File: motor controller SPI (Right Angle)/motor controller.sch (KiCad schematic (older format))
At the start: 27 parts, among them IC1 MA702, IC2 MC33926PNB, IC3 LP38690SD-ADJ_NOPB, J1 Conn_01x06_Male, J2 Conn_01x06_Male, J3 Conn_01x04_Male, M1 Motor_DC, U1 STM32L432KCUx, Y1 32mhz

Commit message: Updated footprints
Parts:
- removed C1, C2: 10pF, Capacitor_SMD:C_0402_1005Metric, symbol Device:C
- removed IC3: LP38690SD-ADJ_NOPB, LP38690SD-ADJ_NOPB:SON95P300X300X80-7N, symbol LP38690SD-ADJ_NOPB:LP38690SD-ADJ_NOPB
- removed Y1: 32mhz, Crystal:Crystal_SMD_2016-4Pin_2.0x1.6mm, symbol Device:Crystal_GND24
- added U2: MIC5501-3.0YM5, Package_TO_SOT_SMD:SOT-23-5, symbol Regulator_Linear:MIC5501-3.0YM5
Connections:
- wire segments 36 -> 28
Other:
- moved on the sheet: C9
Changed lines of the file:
@@
-$EndComp
-$Comp
-L Device:C C1
-U 1 1 5B480489
-P 1000 2650
-F 0 "C1" V 748 2650 50  0000 C CNN
-F 1 "10pF" V 839 2650 50  0000 C CNN
-F 2 "Capacitor_SMD:C_0402_1005Metric" H 1038 2500 50  0001 C CNN
-F 3 "~" H 1000 2650 50  0001 C CNN
-	1    1000 2650
-	0    1    1    0
-$EndComp
-$Comp
-L Device:C C2
-U 1 1 5B480490
-P 1000 2950
-F 0 "C2" V 1252 2950 50  0000 C CNN
-F 1 "10pF" V 1161 2950 50  0000 C CNN
-F 2 "Capacitor_SMD:C_0402_1005Metric" H 1038 2800 50  0001 C CNN
-F 3 "~" H 1000 2950 50  0001 C CNN
-	1    1000 2950
-	0    -1   -1   0
-$EndComp
-Wire Wire Line
-	850  2650 850  2800
-Wire Wire Line
-	1150 2650 1300 2650
-Wire Wire Line
-	1150 2950 1300 2950
-Connection ~ 1300 2950
-Connection ~ 1300 2650
-$Comp
-L power:GND #PWR0101
-U 1 1 5B4804A2
-P 850 2800
-F 0 "#PWR0101" H 850 2550 50  0001 C CNN
-F 1 "GND" V 855 2672 50  0000 R CNN
-F 2 "" H 850 2800 50  0001 C CNN
-F 3 "" H 850 2800 50  0001 C CNN
-	1    850  2800
-	0    1    1    0
-$EndComp
-Connection ~ 850  2800
-Wire Wire Line
-	850  2800 850  2950
-Wire Wire Line
-	1300 2950 2050 2950
-Wire Wire Line
-	1550 2850 2050 2850
-Wire Wire Line
-	1550 2650 1550 2850
-$Comp
-L power:GND #PWR0102
-U 1 1 5B487486
-P 1600 2650
-F 0 "#PWR0102" H 1600 2400 50  0001 C CNN
-F 1 "GND" H 1605 2477 50  0000 C CNN
-F 2 "" H 1600 2650 50  0001 C CNN
-F 3 "" H 1600 2650 50  0001 C CNN
-	1    1600 2650
-	1    0    0    -1
-$EndComp
-$Comp
-L Device:Crystal_GND24 Y1
-U 1 1 5B487B97
-P 1300 2800
-F 0 "Y1" V 1254 3041 50  0000 L CNN
-F 1 "32mhz" V 1345 3041 50  0000 L CNN
-F 2 "Crystal:Crystal_SMD_2016-4Pin_2.0x1.6mm" H 1300 2800 50  0001 C CNN
-F 3 "~" H 1300 2800 50  0001 C CNN
-	1    1300 2800
-	0    1    1    0
-$EndComp
-$Comp
-L power:GND #PWR0131
-U 1 1 5B487CF1
-P 1100 2800
-F 0 "#PWR0131" H 1100 2550 50  0001 C CNN
-F 1 "GND" H 1105 2627 50  0000 C CNN
-F 2 "" H 1100 2800 50  0001 C CNN
-F 3 "" H 1100 2800 50  0001 C CNN
-	1    1100 2800
-	1    0    0    -1
-$EndComp
-$Comp
-L power:GND #PWR0132
-U 1 1 5B487D2A
-P 1500 2800
-F 0 "#PWR0132" H 1500 2550 50  0001 C CNN
-F 1 "GND" H 1505 2627 50  0000 C CNN
-F 2 "" H 1500 2800 50  0001 C CNN
-F 3 "" H 1500 2800 50  0001 C CNN
-	1    1500 2800
-	1    0    0    -1
 $EndComp
 $Comp
@@
 $EndComp
 $Comp
-L LP38690SD-ADJ_NOPB:LP38690SD-ADJ_NOPB IC3
-U 1 1 5B48B2F0
-P 2250 6500
-F 0 "IC3" H 2850 6765 50  0000 C CNN
-F 1 "LP38690SD-ADJ_NOPB" H 2850 6674 50  0000 C CNN
-F 2 "LP38690SD-ADJ_NOPB:SON95P300X300X80-7N" H 3300 6600 50  0001 L CNN
-F 3 "http://uk.rs-online.com/web/p/products/6515542" H 3300 6500 50  0001 L CNN
-F 4 "1A LDO Regulator Adj.,LP38690SD-ADJ Texas Instruments LP38690SD-ADJ/NOPB, LDO Voltage Regulator, Adjustable 1A, 1.25  9 V 2.5%, 6-Pin LLP" H 3300 6400 50  0001 L CNN "Description"
-F 5 "0.8" H 3300 6300 50  0001 L CNN "Height"
-F 6 "Texas Instruments" H 3300 6200 50  0001 L CNN "Manufacturer_Name"
-F 7 "LP38690SD-ADJ/NOPB" H 3300 6100 50  0001 L CNN "Manufacturer_Part_Number"
-F 8 "6515542P" H 3300 6000 50  0001 L CNN "RS Part Number"
-F 9 "http://uk.rs-online.com/web/p/products/6515542P" H 3300 5900 50  0001 L CNN "RS Price/Stock"
-F 10 "LP38690SD-ADJ/NOPB" H 3300 5800 50  0001 L CNN "Arrow Part Number"
-F 11 "https://www.arrow.com/en/products/lp38690sd-adjnopb/texas-instruments" H 3300 5700 50  0001 L CNN "Arrow Price/Stock"
-	1    2250 6500
-	1    0    0    -1
-$EndComp
-$Comp
 L power:+BATT #PWR0139
 U 1 1 5B48B714
@@
 	0    -1   -1   0
 $EndComp
-$Comp
-L power:+BATT #PWR0140
-U 1 1 5B48B7C0
-P 3450 6500
-F 0 "#PWR0140" H 3450 6350 50  0001 C CNN
-F 1 "+BATT" V 3465 6628 50  0000 L CNN
-F 2 "" H 3450 6500 50  0001 C CNN
-F 3 "" H 3450 6500 50  0001 C CNN
-	1    3450 6500
-	0    1    1    0
-$EndComp
-$Comp
-L power:GND #PWR0141
-U 1 1 5B48B8A1
-P 2250 6600
-F 0 "#PWR0141" H 2250 6350 50  0001 C CNN
-F 1 "GND" V 2255 6472 50  0000 R CNN
-F 2 "" H 2250 6600 50  0001 C CNN
-F 3 "" H 2250 6600 50  0001 C CNN
-	1    2250 6600
-	0    1    1    0
-$EndComp
-Wire Wire Line
-	3450 6600 3650 6600
-Wire Wire Line
-	3450 6700 3650 6700
-Wire Wire Line
-	3650 6700 3650 6600
-Connection ~ 3650 6600
-Wire Wire Line
-	3650 6600 3850 6600
+Wire Wire Line
+	3250 6600 3250 6500
+Wire Wire Line
+	3250 6500 3450 6500
 $Comp
 L Device:C C9
 U 1 1 5B48C9E6
-P 3650 6850
-F 0 "C9" H 3765 6896 50  0000 L CNN
-F 1 "1UF" H 3765 6805 50  0000 L CNN
-F 2 "Capacitor_SMD:C_0402_1005Metric" H 3688 6700 50  0001 C CNN
-F 3 "~" H 3650 6850 50  0001 C CNN
-	1    3650 6850
-	1    0    0    -1
-$EndComp
-Connection ~ 3650 6700
+P 3250 6750
+F 0 "C9" H 3365 6796 50  0000 L CNN
+F 1 "1UF" H 3365 6705 50  0000 L CNN
+F 2 "Capacitor_SMD:C_0402_1005Metric" H 3288 6600 50  0001 C CNN
+F 3 "~" H 3250 6750 50  0001 C CNN
+	1    3250 6750
+	1    0    0    -1
+$EndComp
 $Comp
 L Device:C C8
@@
 L power:GND #PWR0143
 U 1 1 5B48CC3C
-P 3650 7000
-F 0 "#PWR0143" H 3650 6750 50  0001 C CNN
-F 1 "GND" H 3655 6827 50  0000 C CNN
-F 2 "" H 3650 7000 50  0001 C CNN
-F 3 "" H 3650 7000 50  0001 C CNN
-	1    3650 7000
+P 3250 6900
+F 0 "#PWR0143" H 3250 6650 50  0001 C CNN
+F 1 "GND" H 3255 6727 50  0000 C CNN
+F 2 "" H 3250 6900 50  0001 C CNN
+F 3 "" H 3250 6900 50  0001 C CNN
+	1    3250 6900
 	1    0    0    -1
 $EndComp
@@
 L power:+3.3V #PWR0144
 U 1 1 5B48CCB0
-P 3850 6600
-F 0 "#PWR0144" H 3850 6450 50  0001 C CNN
-F 1 "+3.3V" V 3865 6728 50  0000 L CNN
-F 2 "" H 3850 6600 50  0001 C CNN
-F 3 "" H 3850 6600 50  0001 C CNN
-	1    3850 6600
+P 3450 6500
+F 0 "#PWR0144" H 3450 6350 50  0001 C CNN
+F 1 "+3.3V" V 3465 6628 50  0000 L CNN
+F 2 "" H 3450 6500 50  0001 C CNN
+F 3 "" H 3450 6500 50  0001 C CNN
+	1    3450 6500
 	0    1    1    0
 $EndComp
@@
 L power:GND #PWR0145
 U 1 1 5B48CD44
-P 2850 7200
-F 0 "#PWR0145" H 2850 6950 50  0001 C CNN
-F 1 "GND" H 2855 7027 50  0000 C CNN
-F 2 "" H 2850 7200 50  0001 C CNN
-F 3 "" H 2850 7200 50  0001 C CNN
-	1    2850 7200
+P 2650 6900
+F 0 "#PWR0145" H 2650 6650 50  0001 C CNN
+F 1 "GND" H 2655 6727 50  0000 C CNN
+F 2 "" H 2650 6900 50  0001 C CNN
+F 3 "" H 2650 6900 50  0001 C CNN
+	1    2650 6900
 	1    0    0    -1
 $EndComp
@@
 Wire Wire Line
 	1900 2650 1800 2650
-Wire Wire Line
-	1300 2650 1550 2650
 Wire Wire Line
 	1900 2650 2050 2650
@@
 Text GLabel 3050 3750 2    50   Input ~ 0
 IN2
+$Comp
+L Regulator_Linear:MIC5501-3.0YM5 U2
+U 1 1 5BABAE39
+P 2650 6600
+F 0 "U2" H 2650 6967 50  0000 C CNN
+F 1 "MIC5501-3.0YM5" H 2650 6876 50  0000 C CNN
+F 2 "Package_TO_SOT_SMD:SOT-23-5" H 2650 6200 50  0001 C CNN
+F 3 "http://ww1.microchip.com/downloads/en/DeviceDoc/MIC550X.pdf" H 2400 6850 50  0001 C CNN
+	1    2650 6600
+	1    0    0    -1
+$EndComp
+Wire Wire Line
+	3050 6500 3250 6500
+Connection ~ 3250 6500
+Wire Wire Line
+	2250 6500 2250 6700
+$Comp
+L power:GND #PWR0101
+U 1 1 5BABFABE
+P 1600 2650
+F 0 "#PWR0101" H 1600 2400 50  0001 C CNN
+F 1 "GND" V 1605 2522 50  0000 R CNN
+F 2 "" H 1600 2650 50  0001 C CNN
+F 3 "" H 1600 2650 50  0001 C CNN
+	1    1600 2650
+	0    1    1    0
+$EndComp
 $EndSCHEMATC

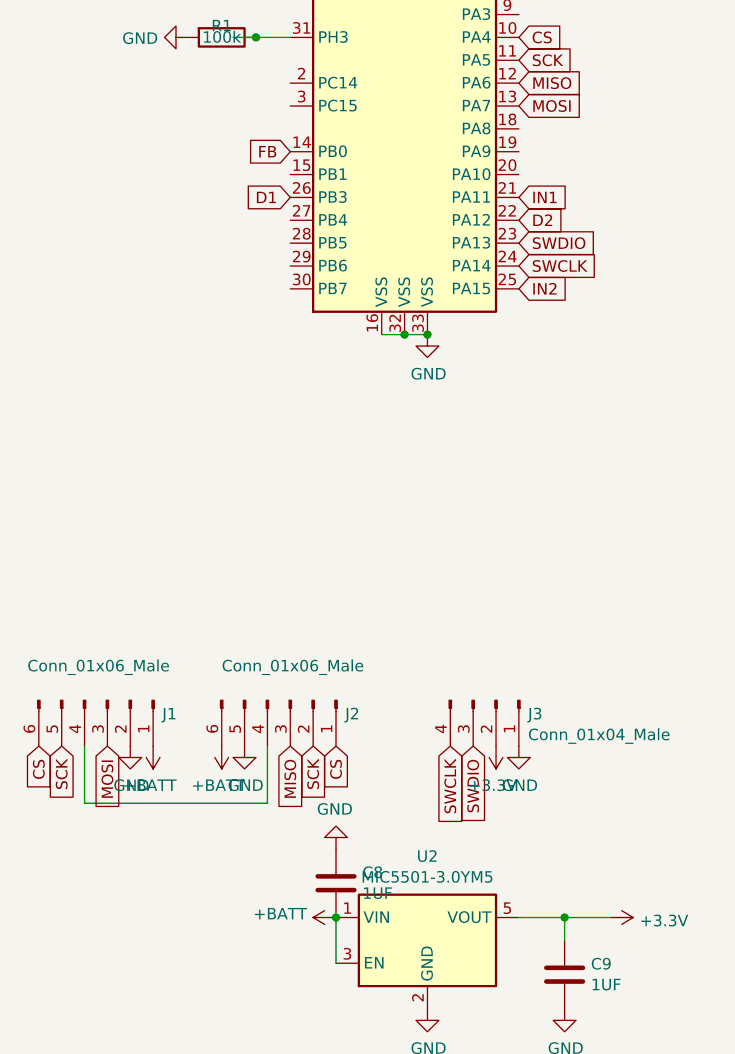
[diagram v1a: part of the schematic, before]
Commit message: Push to new server
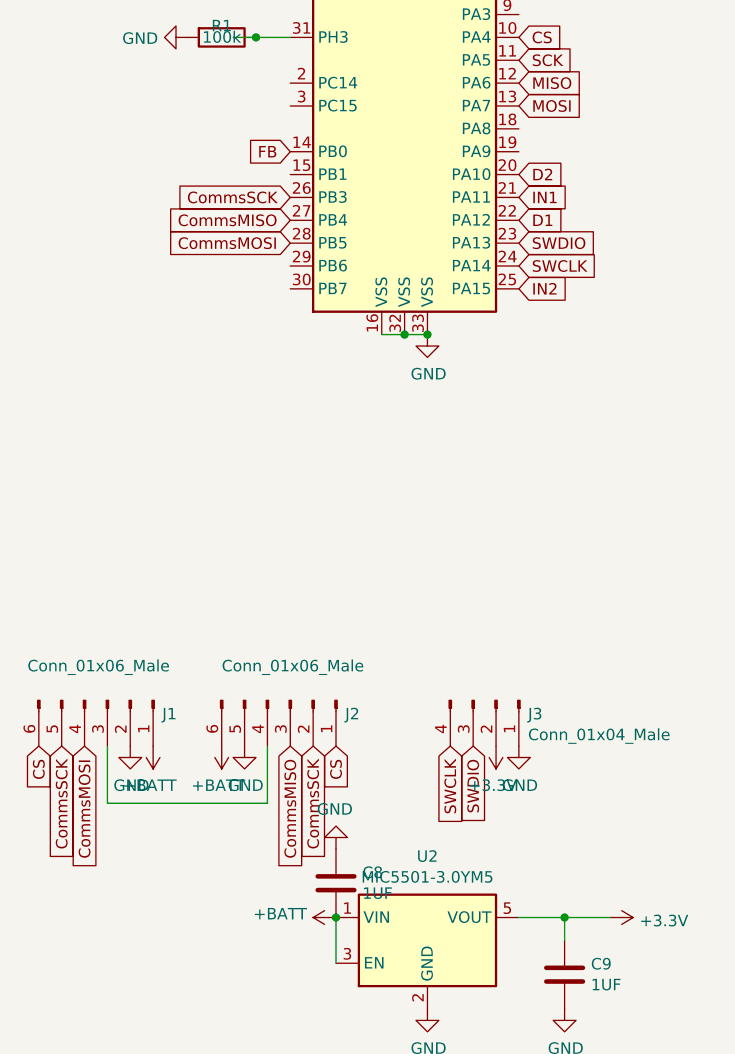
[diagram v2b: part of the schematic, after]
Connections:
- net labels added: CommsMISO, CommsMOSI, CommsSCK
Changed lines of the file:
@@
 Text GLabel 3050 3650 2    50   Input ~ 0
 SWCLK
+Text GLabel 3050 3250 2    50   Input ~ 0
+D2
 Text GLabel 3050 3450 2    50   Input ~ 0
-D2
-Text GLabel 2050 3350 0    50   Input ~ 0
 D1
 $Comp
@@
 	-1   0    0    1
 $EndComp
-Text GLabel 1250 5750 3    50   Input ~ 0
-MOSI
+Text GLabel 1150 5750 3    50   Input ~ 0
+CommsMOSI
 Text GLabel 1050 5750 3    50   Input ~ 0
-SCK
+CommsSCK
 Text GLabel 950  5750 3    50   Input ~ 0
 CS
 Text GLabel 2050 5750 3    50   Input ~ 0
-MISO
+CommsMISO
 Text GLabel 2150 5750 3    50   Input ~ 0
-SCK
+CommsSCK
 Text GLabel 2250 5750 3    50   Input ~ 0
 CS
-Wire Wire Line
-	1150 5750 1150 6000
-Wire Wire Line
-	1150 6000 1950 6000
 $Comp
 L power:+BATT #PWR0133
@@
 	0    1    1    0
 $EndComp
+Text GLabel 2050 3350 0    50   Input ~ 0
+CommsSCK
+Text GLabel 2050 3450 0    50   Input ~ 0
+CommsMISO
+Text GLabel 2050 3550 0    50   Input ~ 0
+CommsMOSI
+Wire Wire Line
+	1250 5750 1250 6000
+Wire Wire Line
+	1250 6000 1950 6000
 $EndSCHEMATC
